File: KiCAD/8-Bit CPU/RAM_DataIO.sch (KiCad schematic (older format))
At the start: 13 parts, among them SW3 SW_DIP_x08, U10 74HC245, U11 74HC245, U9 74HC245

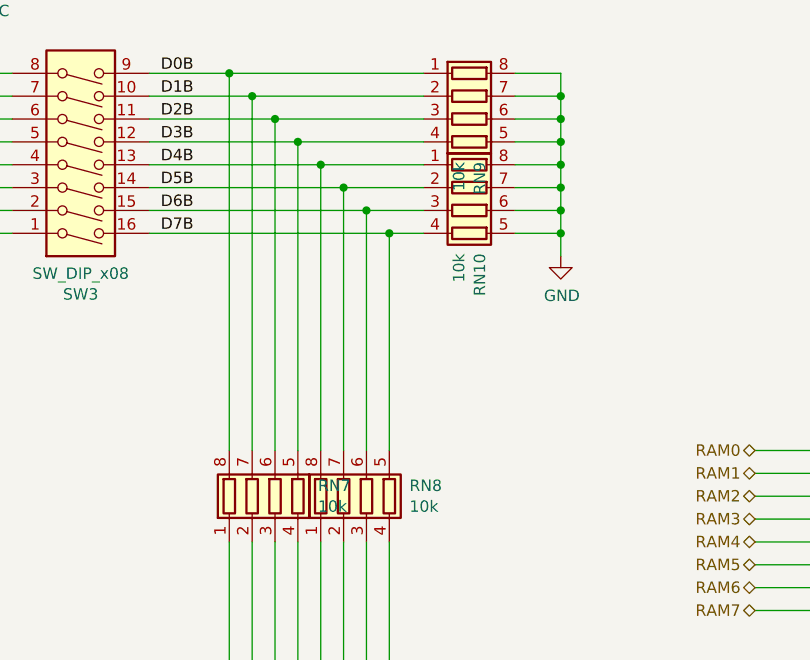
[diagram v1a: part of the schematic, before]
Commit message: KiCAD files update & Gerbers
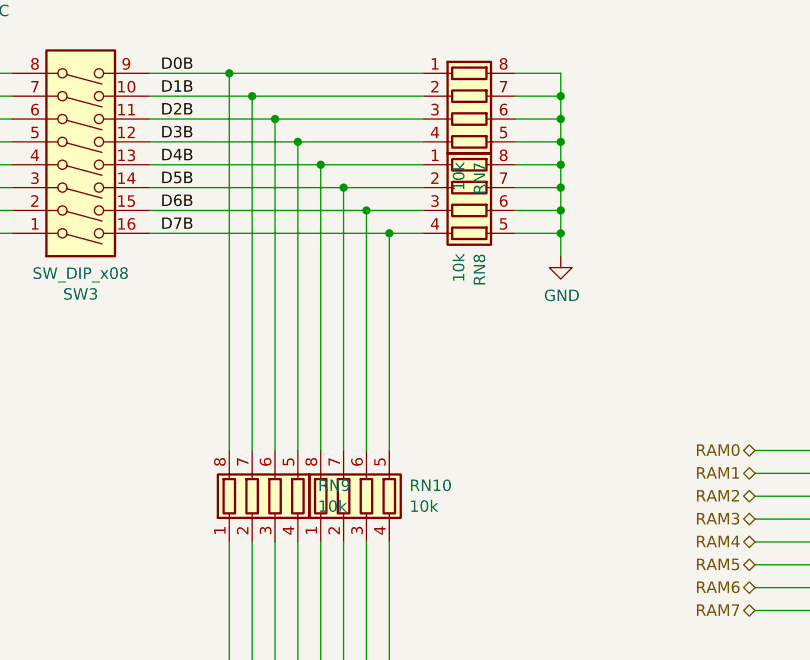
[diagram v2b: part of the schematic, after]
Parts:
- renumbered RN8 to RN10, RN9 to RN7, RN10 to RN8, RN7 to RN9
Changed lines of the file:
@@
 Title ""
 Date ""
-Rev ""
+Rev "C"
 Comp ""
 Comment1 ""
@@
 AR Path="/5D450B31/5D62AA60" Ref="#PWR?"  Part="1"
 AR Path="/5D450B31/5D5C018E/5D62AA60" Ref="#PWR?"  Part="1"
-AR Path="/5D643828/5D450B31/5D62AA60" Ref="#PWR064"  Part="1"
-F 0 "#PWR064" H 7300 5150 50  0001 C CNN
+AR Path="/5D643828/5D450B31/5D62AA60" Ref="#PWR057"  Part="1"
+F 0 "#PWR057" H 7300 5150 50  0001 C CNN
 F 1 "VCC" H 7317 5473 50  0000 C CNN
 F 2 "" H 7300 5300 50  0001 C CNN
@@
 	7250 5000 7750 5000
 $Comp
-L power:VCC #PWR062
+L power:VCC #PWR053
 U 1 1 5D5B189D
 P 6750 4000
-F 0 "#PWR062" H 6750 3850 50  0001 C CNN
+F 0 "#PWR053" H 6750 3850 50  0001 C CNN
 F 1 "VCC" H 6767 4173 50  0000 C CNN
 F 2 "" H 6750 4000 50  0001 C CNN
@@
 $EndComp
 $Comp
-L power:GND #PWR063
+L power:GND #PWR064
 U 1 1 5D4BB0DD
 P 6750 5600
-F 0 "#PWR063" H 6750 5350 50  0001 C CNN
+F 0 "#PWR064" H 6750 5350 50  0001 C CNN
 F 1 "GND" H 6755 5427 50  0000 C CNN
 F 2 "" H 6750 5600 50  0001 C CNN
@@
 $EndComp
 $Comp
-L power:VCC #PWR061
+L power:VCC #PWR054
 U 1 1 5D6A7DF1
 P 6150 5200
-F 0 "#PWR061" H 6150 5050 50  0001 C CNN
+F 0 "#PWR054" H 6150 5050 50  0001 C CNN
 F 1 "VCC" V 6167 5373 50  0000 C CNN
 F 2 "" H 6150 5200 50  0001 C CNN
@@
 AR Path="/5D450B31/5D6E99D0" Ref="#PWR?"  Part="1"
 AR Path="/5D643828/5D5738D6/5D6E99D0" Ref="#PWR?"  Part="1"
-AR Path="/5D643828/5D450B31/5D6E99D0" Ref="#PWR053"  Part="1"
-F 0 "#PWR053" H 1900 5350 50  0001 C CNN
+AR Path="/5D643828/5D450B31/5D6E99D0" Ref="#PWR060"  Part="1"
+F 0 "#PWR060" H 1900 5350 50  0001 C CNN
 F 1 "GND" H 1905 5427 50  0000 C CNN
 F 2 "" H 1900 5600 50  0001 C CNN
@@
 AR Path="/5D450B31/5D6E9D11" Ref="#PWR?"  Part="1"
 AR Path="/5D643828/5D5738D6/5D6E9D11" Ref="#PWR?"  Part="1"
-AR Path="/5D643828/5D450B31/5D6E9D11" Ref="#PWR052"  Part="1"
-F 0 "#PWR052" H 1900 3850 50  0001 C CNN
+AR Path="/5D643828/5D450B31/5D6E9D11" Ref="#PWR051"  Part="1"
+F 0 "#PWR051" H 1900 3850 50  0001 C CNN
 F 1 "VCC" H 1917 4173 50  0000 C CNN
 F 2 "" H 1900 4000 50  0001 C CNN
@@
 AR Path="/5D450B31/5D6EB19A" Ref="#PWR?"  Part="1"
 AR Path="/5D643828/5D5738D6/5D6EB19A" Ref="#PWR?"  Part="1"
-AR Path="/5D643828/5D450B31/5D6EB19A" Ref="#PWR049"  Part="1"
-F 0 "#PWR049" H 1300 5150 50  0001 C CNN
+AR Path="/5D643828/5D450B31/5D6EB19A" Ref="#PWR055"  Part="1"
+F 0 "#PWR055" H 1300 5150 50  0001 C CNN
 F 1 "VCC" H 1317 5473 50  0000 C CNN
 F 2 "" H 1300 5300 50  0001 C CNN
@@
 AR Path="/5D450B31/5D6EB1A0" Ref="#PWR?"  Part="1"
 AR Path="/5D643828/5D5738D6/5D6EB1A0" Ref="#PWR?"  Part="1"
-AR Path="/5D643828/5D450B31/5D6EB1A0" Ref="#PWR050"  Part="1"
-F 0 "#PWR050" H 1300 5350 50  0001 C CNN
+AR Path="/5D643828/5D450B31/5D6EB1A0" Ref="#PWR059"  Part="1"
+F 0 "#PWR059" H 1300 5350 50  0001 C CNN
 F 1 "GND" H 1305 5427 50  0000 C CNN
 F 2 "" H 1300 5600 50  0001 C CNN
@@
 AR Path="/5D450B31/5D91720B" Ref="#PWR?"  Part="1"
 AR Path="/5D643828/5D5738D6/5D91720B" Ref="#PWR?"  Part="1"
-AR Path="/5D643828/5D450B31/5D91720B" Ref="#PWR058"  Part="1"
-F 0 "#PWR058" H 3900 5350 50  0001 C CNN
+AR Path="/5D643828/5D450B31/5D91720B" Ref="#PWR062"  Part="1"
+F 0 "#PWR062" H 3900 5350 50  0001 C CNN
 F 1 "GND" H 3905 5427 50  0000 C CNN
 F 2 "" H 3900 5600 50  0001 C CNN
@@
 AR Path="/5D450B31/5D917211" Ref="#PWR?"  Part="1"
 AR Path="/5D643828/5D5738D6/5D917211" Ref="#PWR?"  Part="1"
-AR Path="/5D643828/5D450B31/5D917211" Ref="#PWR057"  Part="1"
-F 0 "#PWR057" H 3900 3850 50  0001 C CNN
+AR Path="/5D643828/5D450B31/5D917211" Ref="#PWR052"  Part="1"
+F 0 "#PWR052" H 3900 3850 50  0001 C CNN
 F 1 "VCC" H 3917 4173 50  0000 C CNN
 F 2 "" H 3900 4000 50  0001 C CNN
@@
 AR Path="/5D450B31/5D91721D" Ref="#PWR?"  Part="1"
 AR Path="/5D643828/5D5738D6/5D91721D" Ref="#PWR?"  Part="1"
-AR Path="/5D643828/5D450B31/5D91721D" Ref="#PWR055"  Part="1"
-F 0 "#PWR055" H 3300 5150 50  0001 C CNN
+AR Path="/5D643828/5D450B31/5D91721D" Ref="#PWR056"  Part="1"
+F 0 "#PWR056" H 3300 5150 50  0001 C CNN
 F 1 "VCC" H 3317 5473 50  0000 C CNN
 F 2 "" H 3300 5300 50  0001 C CNN
@@
 AR Path="/5D450B31/5D917223" Ref="#PWR?"  Part="1"
 AR Path="/5D643828/5D5738D6/5D917223" Ref="#PWR?"  Part="1"
-AR Path="/5D643828/5D450B31/5D917223" Ref="#PWR056"  Part="1"
-F 0 "#PWR056" H 3300 5350 50  0001 C CNN
+AR Path="/5D643828/5D450B31/5D917223" Ref="#PWR061"  Part="1"
+F 0 "#PWR061" H 3300 5350 50  0001 C CNN
 F 1 "GND" H 3305 5427 50  0000 C CNN
 F 2 "" H 3300 5600 50  0001 C CNN
@@
 AR Path="/5D450B31/5D95EA2A" Ref="#PWR?"  Part="1"
 AR Path="/5D643828/5D5738D6/5D95EA2A" Ref="#PWR?"  Part="1"
-AR Path="/5D643828/5D450B31/5D95EA2A" Ref="#PWR060"  Part="1"
-F 0 "#PWR060" H 4500 5350 50  0001 C CNN
+AR Path="/5D643828/5D450B31/5D95EA2A" Ref="#PWR063"  Part="1"
+F 0 "#PWR063" H 4500 5350 50  0001 C CNN
 F 1 "GND" H 4505 5427 50  0000 C CNN
 F 2 "" H 4500 5600 50  0001 C CNN
@@
 	1550 1050 1550 1150
 $Comp
-L power:VCC #PWR051
+L power:VCC #PWR049
 U 1 1 5D4CD6F1
 P 1550 1050
-F 0 "#PWR051" H 1550 900 50  0001 C CNN
+F 0 "#PWR049" H 1550 900 50  0001 C CNN
 F 1 "VCC" H 1567 1223 50  0000 C CNN
 F 2 "" H 1550 1050 50  0001 C CNN
@@
 AR Path="/5D63B238/5D588993" Ref="RN?"  Part="1"
 AR Path="/5D643828/5D5738D6/5D588993" Ref="RN?"  Part="1"
-AR Path="/5D643828/5D450B31/5D588993" Ref="RN10"  Part="1"
-F 0 "RN10" H 3838 1796 50  0000 L CNN
+AR Path="/5D643828/5D450B31/5D588993" Ref="RN8"  Part="1"
+F 0 "RN8" H 3838 1796 50  0000 L CNN
 F 1 "10k" H 3838 1705 50  0000 L CNN
 F 2 "Resistor_SMD:R_Array_Concave_4x0603" V 3925 1750 50  0001 C CNN
@@
 AR Path="/5D63B238/5D58898D" Ref="RN?"  Part="1"
 AR Path="/5D643828/5D5738D6/5D58898D" Ref="RN?"  Part="1"
-AR Path="/5D643828/5D450B31/5D58898D" Ref="RN9"  Part="1"
-F 0 "RN9" H 3838 1396 50  0000 L CNN
+AR Path="/5D643828/5D450B31/5D58898D" Ref="RN7"  Part="1"
+F 0 "RN7" H 3838 1396 50  0000 L CNN
 F 1 "10k" H 3838 1305 50  0000 L CNN
 F 2 "Resistor_SMD:R_Array_Concave_4x0603" V 3925 1350 50  0001 C CNN
@@
 AR Path="/5D450B31/5D58897F" Ref="#PWR?"  Part="1"
 AR Path="/5D643828/5D5738D6/5D58897F" Ref="#PWR?"  Part="1"
-AR Path="/5D643828/5D450B31/5D58897F" Ref="#PWR059"  Part="1"
-F 0 "#PWR059" H 4050 1700 50  0001 C CNN
+AR Path="/5D643828/5D450B31/5D58897F" Ref="#PWR050"  Part="1"
+F 0 "#PWR050" H 4050 1700 50  0001 C CNN
 F 1 "GND" H 4055 1777 50  0000 C CNN
 F 2 "" H 4050 1950 50  0001 C CNN
@@
 AR Path="/5D63B238/5D92E498" Ref="RN?"  Part="1"
 AR Path="/5D643828/5D5738D6/5D92E498" Ref="RN?"  Part="1"
-AR Path="/5D643828/5D450B31/5D92E498" Ref="RN7"  Part="1"
-F 0 "RN7" H 2988 3046 50  0000 L CNN
+AR Path="/5D643828/5D450B31/5D92E498" Ref="RN9"  Part="1"
+F 0 "RN9" H 2988 3046 50  0000 L CNN
 F 1 "10k" H 2988 2955 50  0000 L CNN
 F 2 "Resistor_SMD:R_Array_Concave_4x0603" V 3075 3000 50  0001 C CNN
@@
 AR Path="/5D63B238/5D92F51B" Ref="RN?"  Part="1"
 AR Path="/5D643828/5D5738D6/5D92F51B" Ref="RN?"  Part="1"
-AR Path="/5D643828/5D450B31/5D92F51B" Ref="RN8"  Part="1"
-F 0 "RN8" H 3388 3046 50  0000 L CNN
+AR Path="/5D643828/5D450B31/5D92F51B" Ref="RN10"  Part="1"
+F 0 "RN10" H 3388 3046 50  0000 L CNN
 F 1 "10k" H 3388 2955 50  0000 L CNN
 F 2 "Resistor_SMD:R_Array_Concave_4x0603" V 3475 3000 50  0001 C CNN
@@
 AR Path="/5D450B31/5DBA6D3B" Ref="#PWR?"  Part="1"
 AR Path="/5D643828/5D5738D6/5DBA6D3B" Ref="#PWR?"  Part="1"
-AR Path="/5D643828/5D450B31/5DBA6D3B" Ref="#PWR054"  Part="1"
-F 0 "#PWR054" H 2500 5250 50  0001 C CNN
+AR Path="/5D643828/5D450B31/5DBA6D3B" Ref="#PWR058"  Part="1"
+F 0 "#PWR058" H 2500 5250 50  0001 C CNN
 F 1 "GND" H 2505 5327 50  0000 C CNN
 F 2 "" H 2500 5500 50  0001 C CNN
